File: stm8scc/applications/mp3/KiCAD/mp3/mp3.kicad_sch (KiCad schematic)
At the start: 23 parts, among them J1 SD_Card, J2 earphone, SW1 PLAY/STOP, SW2 INC., SW3 DEC., U1 STM8S105C6, Y1 24.576MHz

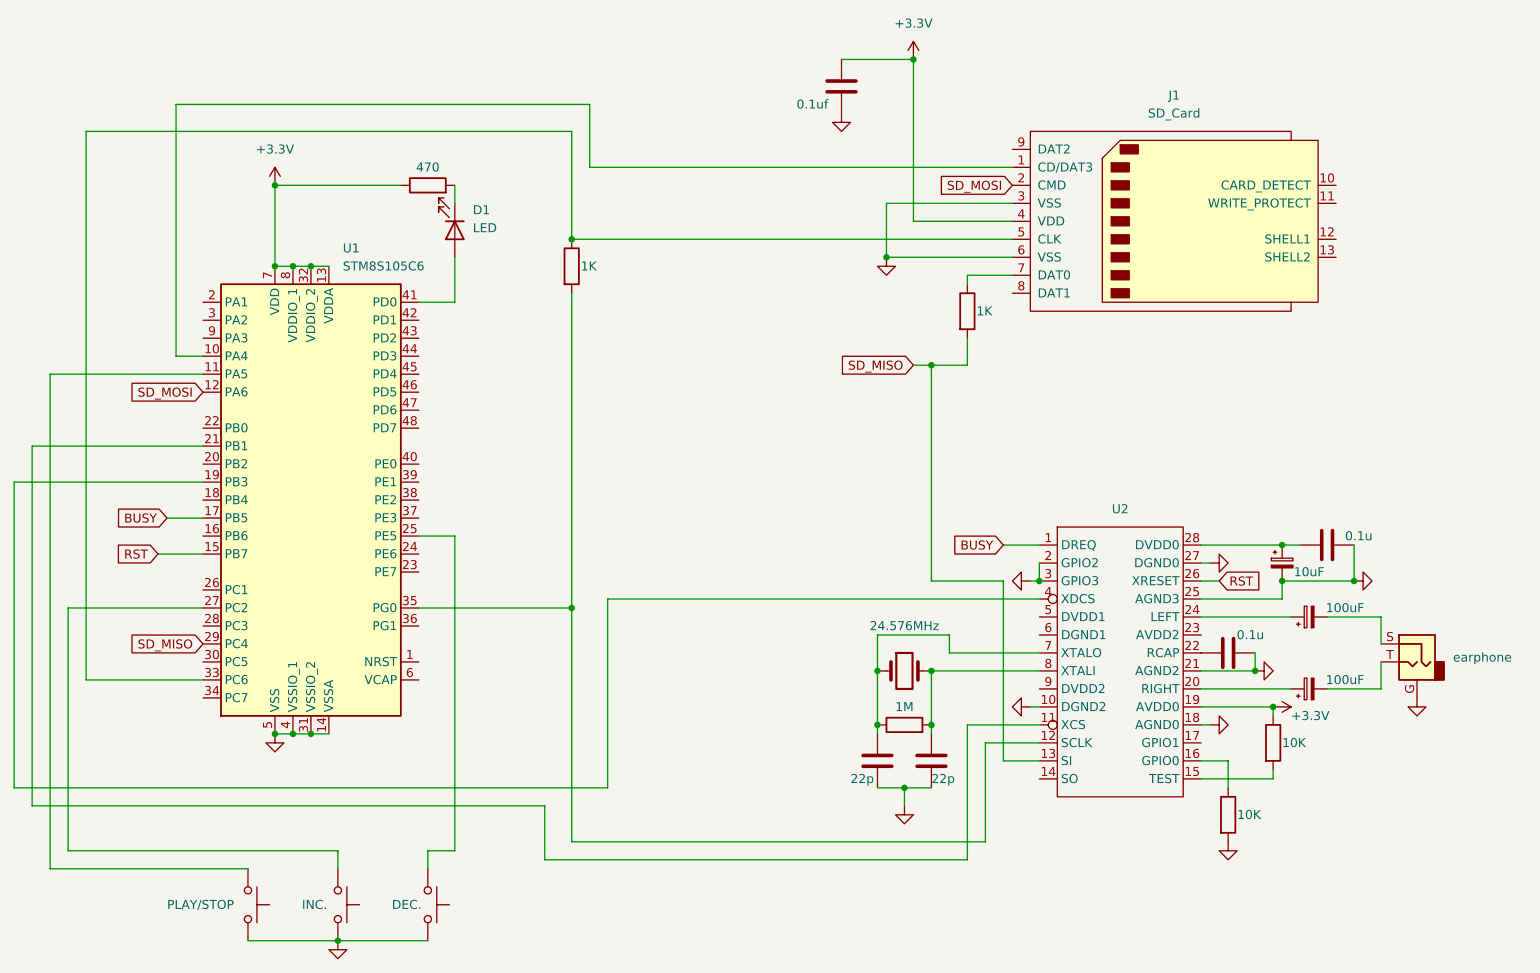
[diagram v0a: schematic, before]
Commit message: ewmove backups
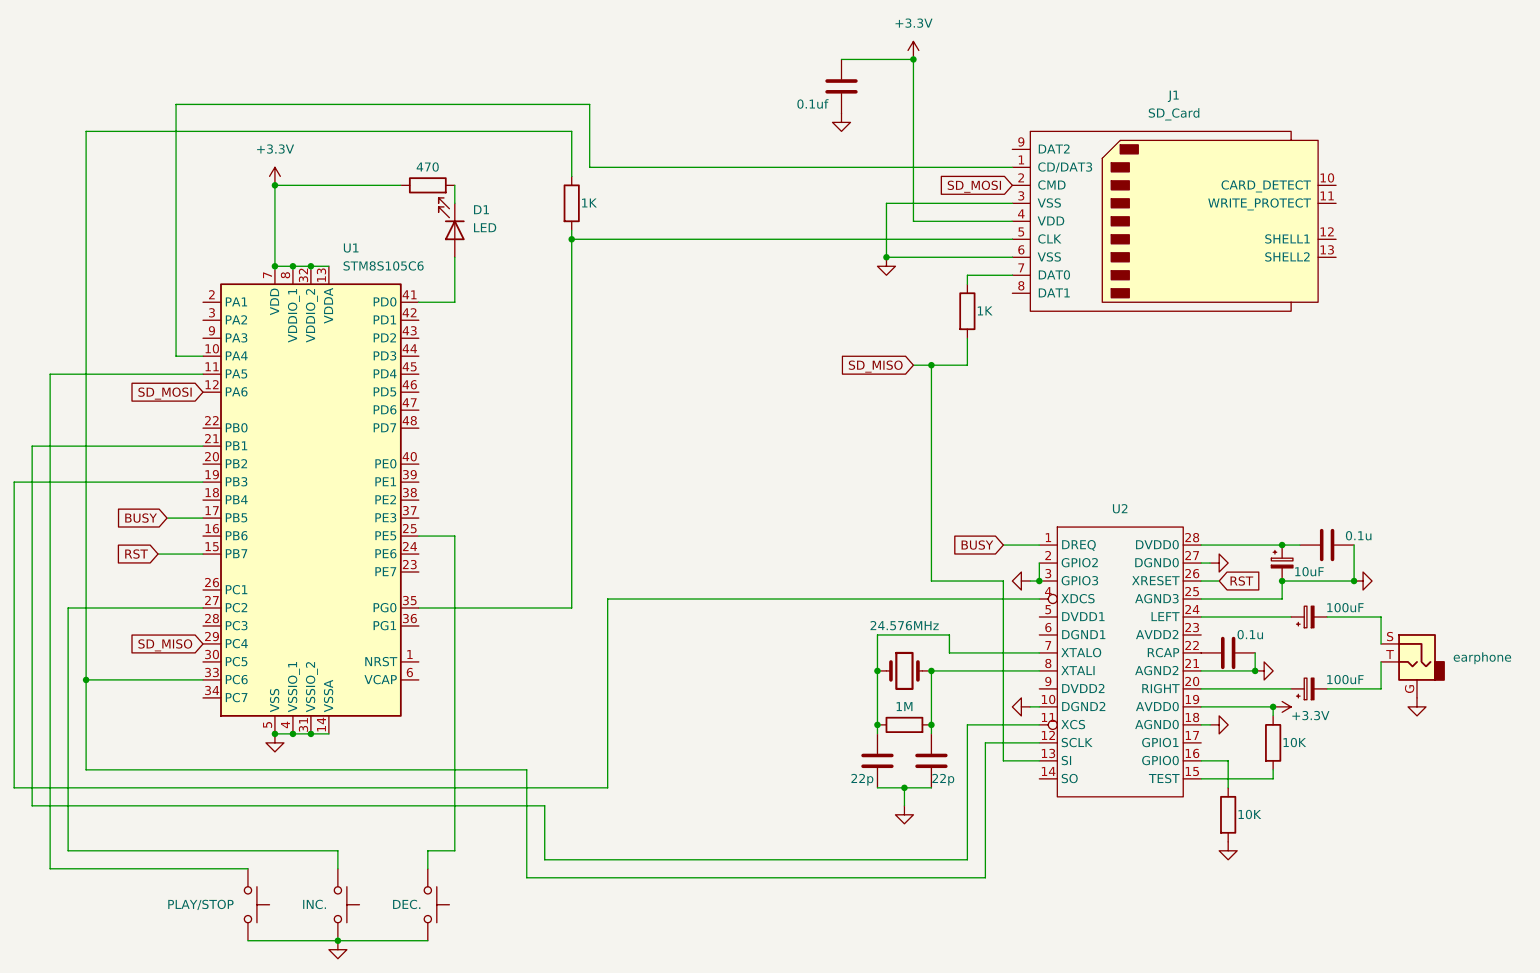
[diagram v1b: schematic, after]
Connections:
- net at R3.1, U1.33 (PC6): now also U2.12 (SCLK); no longer J1.5 (CLK)
- net at R3.2, U1.35 (PG0): now also J1.5 (CLK); no longer U2.12 (SCLK)

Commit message: recover
recover
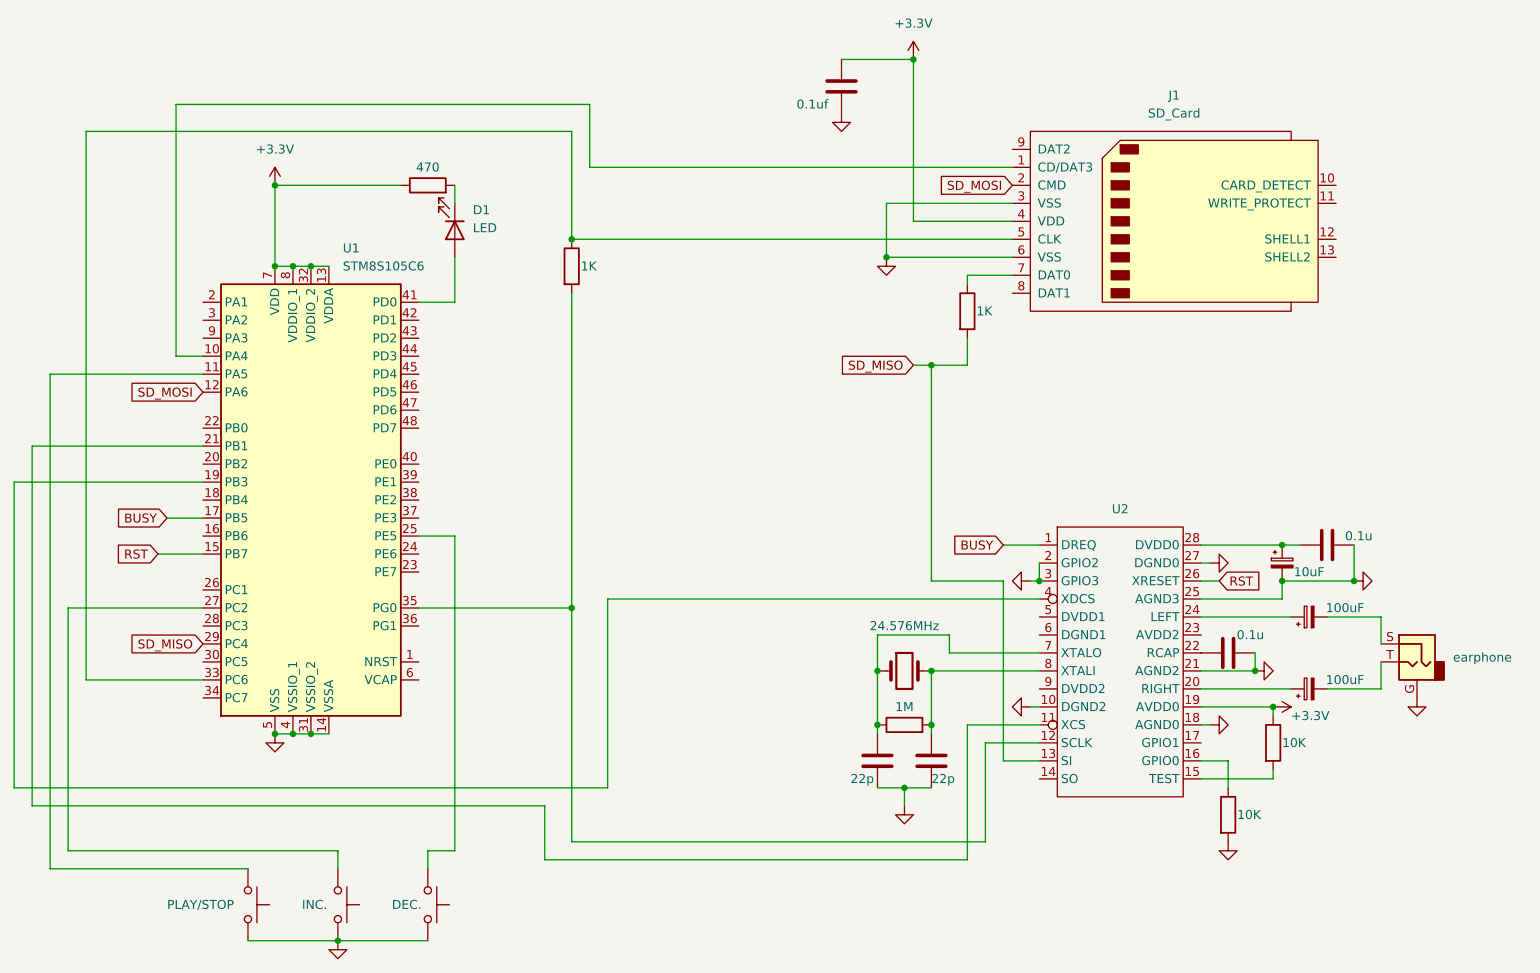
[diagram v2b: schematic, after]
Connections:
- net at R3.2, U1.35 (PG0): now also U2.12 (SCLK); no longer J1.5 (CLK)
- net at R3.1, U1.33 (PC6): now also J1.5 (CLK); no longer U2.12 (SCLK)
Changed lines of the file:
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@@
   (junction (at 156.21 137.16) (diameter 0) (color 0 0 0 0)
   )
+  (junction (at 219.71 107.95) (diameter 0) (color 0 0 0 0)
+  )
+  (junction (at 153.67 62.23) (diameter 0) (color 0 0 0 0)
+  )
+  (junction (at 152.4 128.27) (diameter 0) (color 0 0 0 0)
+  )
+  (junction (at 160.02 120.65) (diameter 0) (color 0 0 0 0)
+  )
+  (junction (at 152.4 120.65) (diameter 0) (color 0 0 0 0)
+  )
   (junction (at 109.22 59.69) (diameter 0) (color 0 0 0 0)
   )
-  (junction (at 219.71 107.95) (diameter 0) (color 0 0 0 0)
-  )
-  (junction (at 153.67 62.23) (diameter 0) (color 0 0 0 0)
-  )
-  (junction (at 152.4 128.27) (diameter 0) (color 0 0 0 0)
-  )
-  (junction (at 160.02 120.65) (diameter 0) (color 0 0 0 0)
-  )
-  (junction (at 152.4 120.65) (diameter 0) (color 0 0 0 0)
-  )
   (junction (at 72.39 129.54) (diameter 0) (color 0 0 0 0)
   )
-  (junction (at 40.64 121.92) (diameter 0) (color 0 0 0 0)
-  )
   (junction (at 69.85 129.54) (diameter 0) (color 0 0 0 0)
   )
@@
   (junction (at 67.31 52.07) (diameter 0) (color 0 0 0 0)
   )
+  (junction (at 109.22 111.76) (diameter 0) (color 0 0 0 0)
+  )
   (junction (at 175.26 107.95) (diameter 0) (color 0 0 0 0)
   )
@@
     (stroke (width 0) (type default))
   )
-  (wire (pts (xy 40.64 134.62) (xy 40.64 121.92))
-    (stroke (width 0) (type default))
-  )
   (wire (pts (xy 165.1 77.47) (xy 160.02 77.47))
     (stroke (width 0) (type default))
@@
     (stroke (width 0) (type default))
   )
+  (wire (pts (xy 87.63 111.76) (xy 109.22 111.76))
+    (stroke (width 0) (type default))
+  )
   (wire (pts (xy 167.64 130.81) (xy 175.26 130.81))
     (stroke (width 0) (type default))
@@
     (stroke (width 0) (type default))
   )
-  (wire (pts (xy 109.22 58.42) (xy 109.22 59.69))
-    (stroke (width 0) (type default))
-  )
   (wire (pts (xy 219.71 107.95) (xy 219.71 102.87))
     (stroke (width 0) (type default))
@@
     (stroke (width 0) (type default))
   )
-  (wire (pts (xy 102.87 149.86) (xy 167.64 149.86))
-    (stroke (width 0) (type default))
-  )
-  (wire (pts (xy 102.87 149.86) (xy 102.87 134.62))
+  (wire (pts (xy 109.22 144.78) (xy 167.64 144.78))
     (stroke (width 0) (type default))
   )
@@
     (stroke (width 0) (type default))
   )
-  (wire (pts (xy 102.87 134.62) (xy 40.64 134.62))
-    (stroke (width 0) (type default))
-  )
   (wire (pts (xy 30.48 137.16) (xy 30.48 93.98))
     (stroke (width 0) (type default))
@@
     (stroke (width 0) (type default))
   )
-  (wire (pts (xy 167.64 149.86) (xy 167.64 130.81))
+  (wire (pts (xy 167.64 144.78) (xy 167.64 130.81))
     (stroke (width 0) (type default))
   )
@@
     (stroke (width 0) (type default))
   )
+  (wire (pts (xy 109.22 111.76) (xy 109.22 144.78))
+    (stroke (width 0) (type default))
+  )
   (wire (pts (xy 153.67 54.61) (xy 153.67 62.23))
     (stroke (width 0) (type default))
@@
     (stroke (width 0) (type default))
   )
-  (wire (pts (xy 109.22 59.69) (xy 109.22 111.76))
-    (stroke (width 0) (type default))
-  )
   (wire (pts (xy 87.63 68.58) (xy 92.71 68.58))
     (stroke (width 0) (type default))
@@
     (stroke (width 0) (type default))
   )
-  (wire (pts (xy 109.22 44.45) (xy 109.22 50.8))
+  (wire (pts (xy 109.22 44.45) (xy 109.22 59.69))
     (stroke (width 0) (type default))
   )
@@
     (stroke (width 0) (type default))
   )
+  (wire (pts (xy 109.22 67.31) (xy 109.22 111.76))
+    (stroke (width 0) (type default))
+  )
   (wire (pts (xy 53.34 40.64) (xy 53.34 76.2))
     (stroke (width 0) (type default))
@@
   )
   (wire (pts (xy 35.56 78.74) (xy 35.56 148.59))
-    (stroke (width 0) (type default))
-  )
-  (wire (pts (xy 87.63 111.76) (xy 109.22 111.76))
     (stroke (width 0) (type default))
   )
@@
     )
   )
-  (symbol (lib_id "Device:R") (at 109.22 54.61 0) (unit 1)
-    (in_bom yes) (on_board yes) (dnp no)
-    (property "Reference" "R3" (at 111.76 53.34 0)
+  (symbol (lib_id "Device:R") (at 109.22 63.5 0) (unit 1)
+    (in_bom yes) (on_board yes) (dnp no)
+    (property "Reference" "R3" (at 111.76 62.23 0)
       (effects (font (size 1.27 1.27)) (justify left) hide)
     )
-    (property "Value" "1K" (at 110.49 54.61 0)
-      (effects (font (size 1.27 1.27)) (justify left))
-    )
-    (property "Footprint" "" (at 107.442 54.61 90)
-      (effects (font (size 1.27 1.27)) hide)
-    )
-    (property "Datasheet" "~" (at 109.22 54.61 0)
-      (effects (font (size 1.27 1.27)) hide)
-    )
+    (property "Value" "1K" (at 110.49 63.5 0)
+      (effects (font (size 1.27 1.27)) (justify left))
+    )
+    (property "Footprint" "" (at 107.442 63.5 90)
+      (effects (font (size 1.27 1.27)) hide)
+    )
+    (property "Datasheet" "~" (at 109.22 63.5 0)
+      (effects (font (size 1.27 1.27)) hide)
+    )
